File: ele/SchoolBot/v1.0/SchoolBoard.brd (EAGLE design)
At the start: 95 x 60 mm, 55 parts, among them X1 M8, X2 M8, X4 POWER_IN

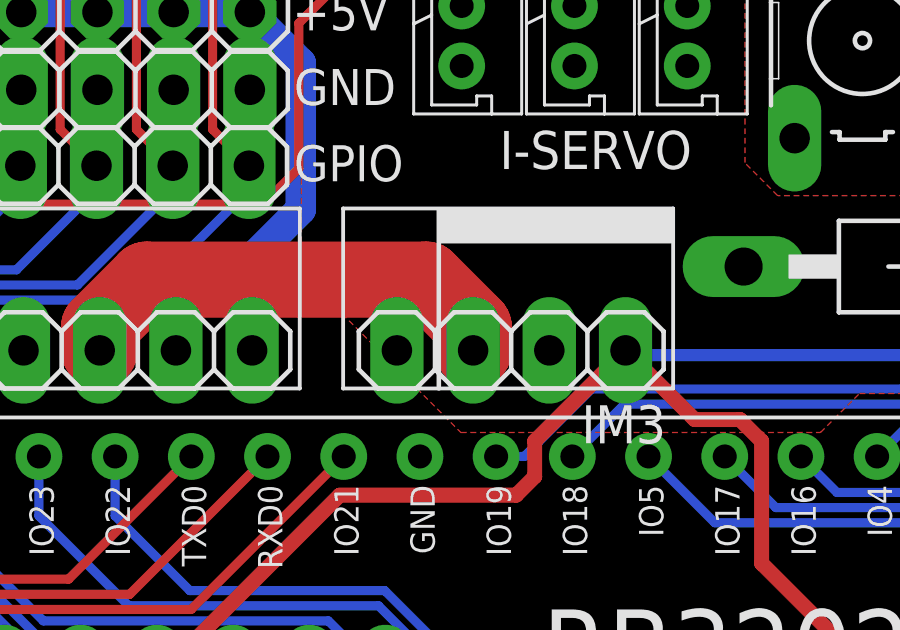
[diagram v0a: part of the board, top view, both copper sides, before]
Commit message: dalsi_text_a_firstbot
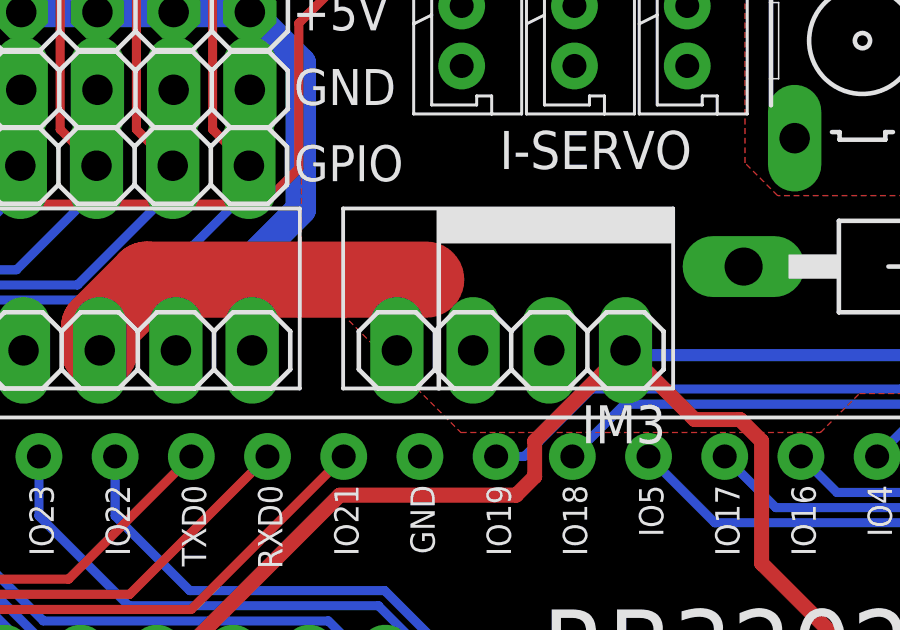
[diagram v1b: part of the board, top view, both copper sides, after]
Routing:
- net VCC: track 71.4 -> 68.4 mm
